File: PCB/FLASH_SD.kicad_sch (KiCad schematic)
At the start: 13 parts, among them J1 MEM2090-00-145-00-A_REVA, U6 HSP051-4M10, U7 HSP051-4M10

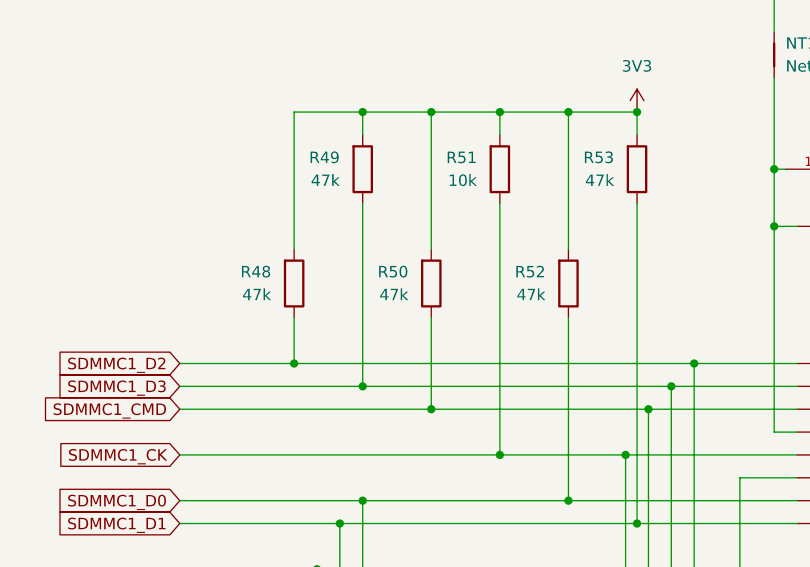
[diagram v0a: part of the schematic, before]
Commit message: update
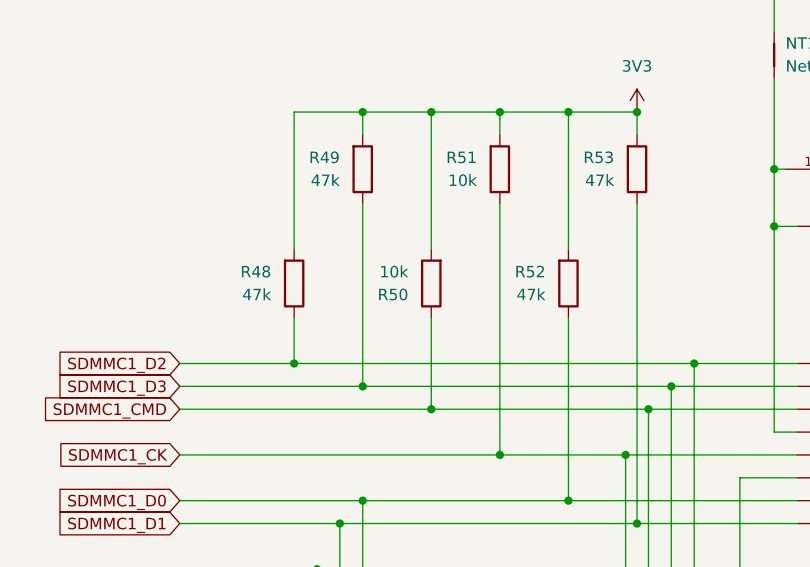
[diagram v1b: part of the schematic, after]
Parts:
- R50: value 47k -> 10k; LCSC Part # C25792 -> C25744
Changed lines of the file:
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@@
+	)
+	(symbol
+		(lib_id "Device:R")
+		(at 307.34 121.92 180)
+		(unit 1)
+		(exclude_from_sim no)
+		(in_bom yes)
+		(on_board yes)
+		(dnp no)
+		(property "Reference" "R50"
+			(at 304.8 123.1901 0)
+			(effects
+				(font
+					(size 1.27 1.27)
+				)
+				(justify left)
+			)
+		)
+		(property "Value" "10k"
+			(at 304.8 120.6501 0)
+			(effects
+				(font
+					(size 1.27 1.27)
+				)
+				(justify left)
+			)
+		)
+		(property "Footprint" "Resistor_SMD:R_0402_1005Metric"
+			(at 309.118 121.92 90)
+			(effects
+				(font
+					(size 1.27 1.27)
+				)
+				(hide yes)
+			)
+		)
+		(property "Datasheet" "~"
+			(at 307.34 121.92 0)
+			(effects
+				(font
+					(size 1.27 1.27)
+				)
+				(hide yes)
+			)
+		)
+		(property "Description" "Resistor"
+			(at 307.34 121.92 0)
+			(effects
+				(font
+					(size 1.27 1.27)
+				)
+				(hide yes)
+			)
+		)
+		(property "Mouser P/N" ""
+			(at 307.34 121.92 0)
+			(effects
+				(font
+					(size 1.27 1.27)
+				)
+				(hide yes)
+			)
+		)
+		(property "BUILT_BY" ""
+			(at 307.34 121.92 90)
+			(effects
+				(font
+					(size 1.27 1.27)
+				)
+				(hide yes)
+			)
+		)
+		(property "COPYRIGHT" ""
+			(at 307.34 121.92 90)
+			(effects
+				(font
+					(size 1.27 1.27)
+				)
+				(hide yes)
+			)
+		)
+		(property "LCSC Part #" "C25744"
+			(at 307.34 121.92 90)
+			(effects
+				(font
+					(size 1.27 1.27)
+				)
+				(hide yes)
+			)
+		)
+		(property "MANUFACTURER_PART_NUMBER" ""
+			(at 307.34 121.92 90)
+			(effects
+				(font
+					(size 1.27 1.27)
+				)
+				(hide yes)
+			)
+		)
+		(property "SNAPEDA_PN" ""
+			(at 307.34 121.92 90)
+			(effects
+				(font
+					(size 1.27 1.27)
+				)
+				(hide yes)
+			)
+		)
+		(property "SOURCELIBRARY" ""
+			(at 307.34 121.92 90)
+			(effects
+				(font
+					(size 1.27 1.27)
+				)
+				(hide yes)
+			)
+		)
+		(property "VENDOR" ""
+			(at 307.34 121.92 90)
+			(effects
+				(font
+					(size 1.27 1.27)
+				)
+				(hide yes)
+			)
+		)
+		(pin "1"
+		)
+		(pin "2"
+		)
+		(instances
+			(project "MPU_MOD"
+				(path "/65890f61-d586-475b-928a-b635a5e4e59e/ec317a3c-922b-4ac6-af1a-f2cdb70bc7c5"
+					(reference "R50")
+					(unit 1)
+				)
+			)
+		)
 	)
 	(symbol
@@
 					(unit 1)
 				)
-			)
-		)
-	)
-	(symbol
-		(lib_id "Device:R")
-		(at 307.34 121.92 0)
-		(mirror x)
-		(unit 1)
-		(exclude_from_sim no)
-		(in_bom yes)
-		(on_board yes)
-		(dnp no)
-		(fields_autoplaced yes)
-		(property "Reference" "R50"
-			(at 304.8 120.6499 0)
-			(effects
-				(font
-					(size 1.27 1.27)
-				)
-				(justify right)
-			)
-		)
-		(property "Value" "47k"
-			(at 304.8 123.1899 0)
-			(effects
-				(font
-					(size 1.27 1.27)
-				)
-				(justify right)
-			)
-		)
-		(property "Footprint" "Resistor_SMD:R_0402_1005Metric"
-			(at 305.562 121.92 90)
-			(effects
-				(font
-					(size 1.27 1.27)
-				)
-				(hide yes)
-			)
-		)
-		(property "Datasheet" "~"
-			(at 307.34 121.92 0)
-			(effects
-				(font
-					(size 1.27 1.27)
-				)
-				(hide yes)
-			)
-		)
-		(property "Description" "Resistor"
-			(at 307.34 121.92 0)
-			(effects
-				(font
-					(size 1.27 1.27)
-				)
-				(hide yes)
-			)
-		)
-		(property "Mouser P/N" ""
-			(at 307.34 121.92 0)
-			(effects
-				(font
-					(size 1.27 1.27)
-				)
-				(hide yes)
-			)
-		)
-		(property "BUILT_BY" ""
-			(at 307.34 121.92 0)
-			(effects
-				(font
-					(size 1.27 1.27)
-				)
-				(hide yes)
-			)
-		)
-		(property "COPYRIGHT" ""
-			(at 307.34 121.92 0)
-			(effects
-				(font
-					(size 1.27 1.27)
-				)
-				(hide yes)
-			)
-		)
-		(property "LCSC Part #" "C25792"
-			(at 307.34 121.92 0)
-			(effects
-				(font
-					(size 1.27 1.27)
-				)
-				(hide yes)
-			)
-		)
-		(property "MANUFACTURER_PART_NUMBER" ""
-			(at 307.34 121.92 0)
-			(effects
-				(font
-					(size 1.27 1.27)
-				)
-				(hide yes)
-			)
-		)
-		(property "SNAPEDA_PN" ""
-			(at 307.34 121.92 0)
-			(effects
-				(font
-					(size 1.27 1.27)
-				)
-				(hide yes)
-			)
-		)
-		(property "SOURCELIBRARY" ""
-			(at 307.34 121.92 0)
-			(effects
-				(font
-					(size 1.27 1.27)
-				)
-				(hide yes)
-			)
-		)
-		(property "VENDOR" ""
-			(at 307.34 121.92 0)
-			(effects
-				(font
-					(size 1.27 1.27)
-				)
-				(hide yes)
-			)
-		)
-		(pin "1"
-		)
-		(pin "2"
-		)
-		(instances
-			(project "MPU_MOD"
-				(path "/65890f61-d586-475b-928a-b635a5e4e59e/ec317a3c-922b-4ac6-af1a-f2cdb70bc7c5"
-					(reference "R50")
-					(unit 1)
-				)
